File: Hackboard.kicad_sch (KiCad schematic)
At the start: 71 parts, among them J1 Conn_01x23_Socket, J2 Micro_SD_Card, J3 Conn_01x31_Socket, J4 Conn_01x08_Socket, J5 Conn_01x02_Pin, J6 USB_C_Receptacle_USB2.0_16P, J7 Barrel_Jack_Switch, Q1 NMOS, Q2 NMOS, Q3 NMOS, SW1 SW_SPST, U1 NCP164CSN330T1G, U2 AP63205WU, U3 STM32L476RGT6, U4 74LVC4245APW, U5 74LVC4245APW, U6 74LVC4245APW, U7 USBLC6-2SC6, U8 74LVC4245APW, U9 74LVC4245APW

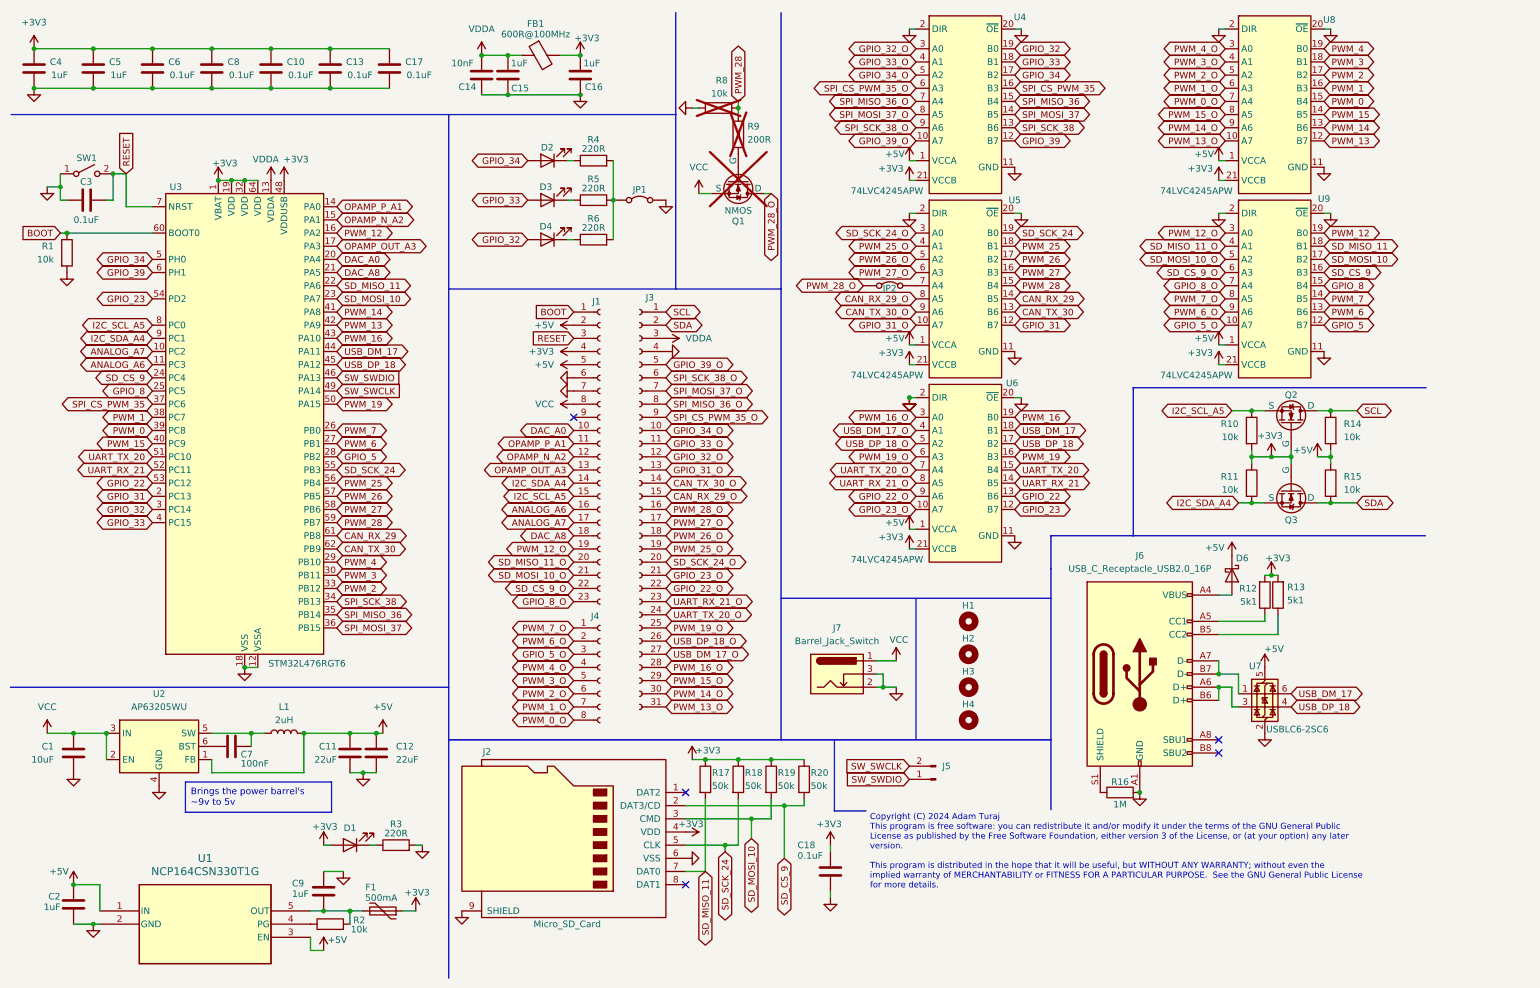
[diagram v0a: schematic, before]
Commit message: Adjust pinout
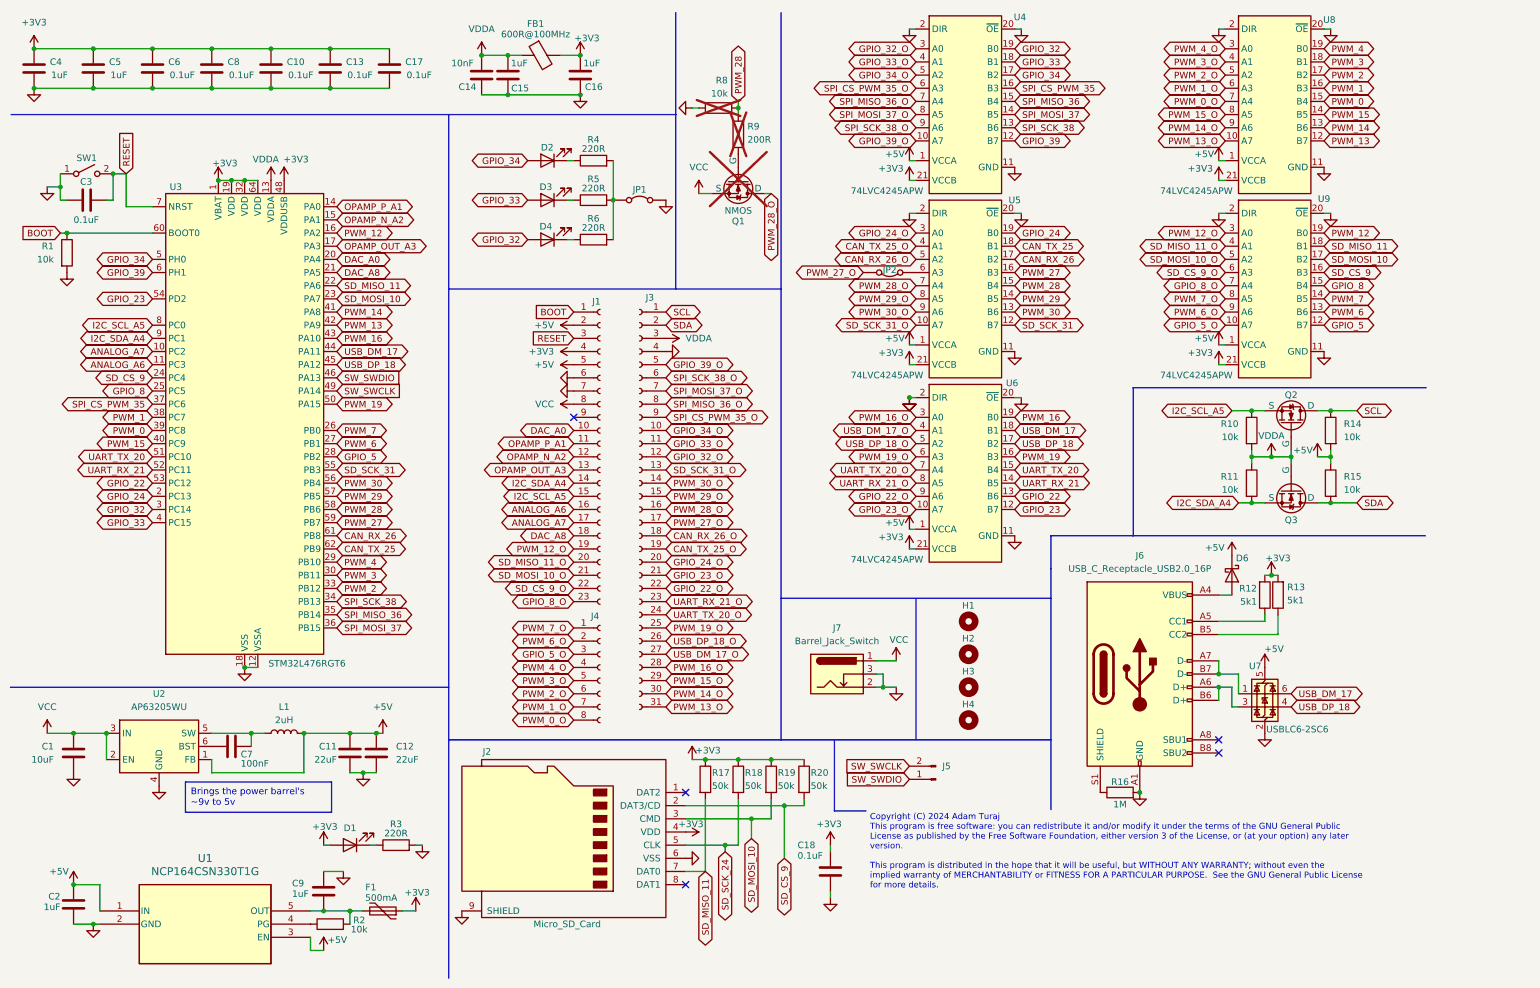
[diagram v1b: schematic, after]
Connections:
- net +3V3: no longer Q2.2 (G), Q3.2 (G), R10.2, R11.1
- net PWM_27: now also U3.59 (PB7); no longer U3.58 (PB6)
- net PWM_27_O: now also JP2.1 (A); no longer U5.6 (A3)
- net PWM_28: now also U3.58 (PB6); no longer U3.59 (PB7)
- net PWM_28_O: now also U5.7 (A4); no longer JP2.1 (A)
- net SD_SCK_24: no longer U3.55 (PB3), U5.19 (B0)
- net VDDA: now also Q2.2 (G), Q3.2 (G), R10.2, R11.1
- net at JP2.2 (B): now also U5.6 (A3); no longer U5.7 (A4)
- net CAN_RX_29 renamed CAN_RX_26
- net CAN_RX_26: now also U5.17 (B2); no longer U5.14 (B5)
- net CAN_RX_29_O renamed PWM_29_O
- net CAN_TX_30 renamed CAN_TX_25
- net CAN_TX_25: now also U5.18 (B1); no longer U5.13 (B6)
- net CAN_TX_30_O renamed PWM_30_O
- net GPIO_31 renamed GPIO_24
- net GPIO_24: now also U5.19 (B0); no longer U5.12 (B7)
- net GPIO_31_O renamed SD_SCK_31_O
- net PWM_25 renamed PWM_30
- net PWM_30: now also U5.13 (B6); no longer U5.18 (B1)
- net PWM_25_O renamed CAN_TX_25_O
- net PWM_26 renamed PWM_29
- net PWM_29: now also U5.14 (B5); no longer U5.17 (B2)
- net PWM_26_O renamed CAN_RX_26_O
- net SD_SCK_24_O renamed GPIO_24_O
- new net SD_SCK_31: U3.55 (PB3), U5.12 (B7)
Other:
- moved on the sheet: JP2
